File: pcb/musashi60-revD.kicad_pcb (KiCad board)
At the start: 2 copper layers, 160 x 135 mm, 68 parts, among them J1 MJ-4PP-9, U1 ProMicro_r

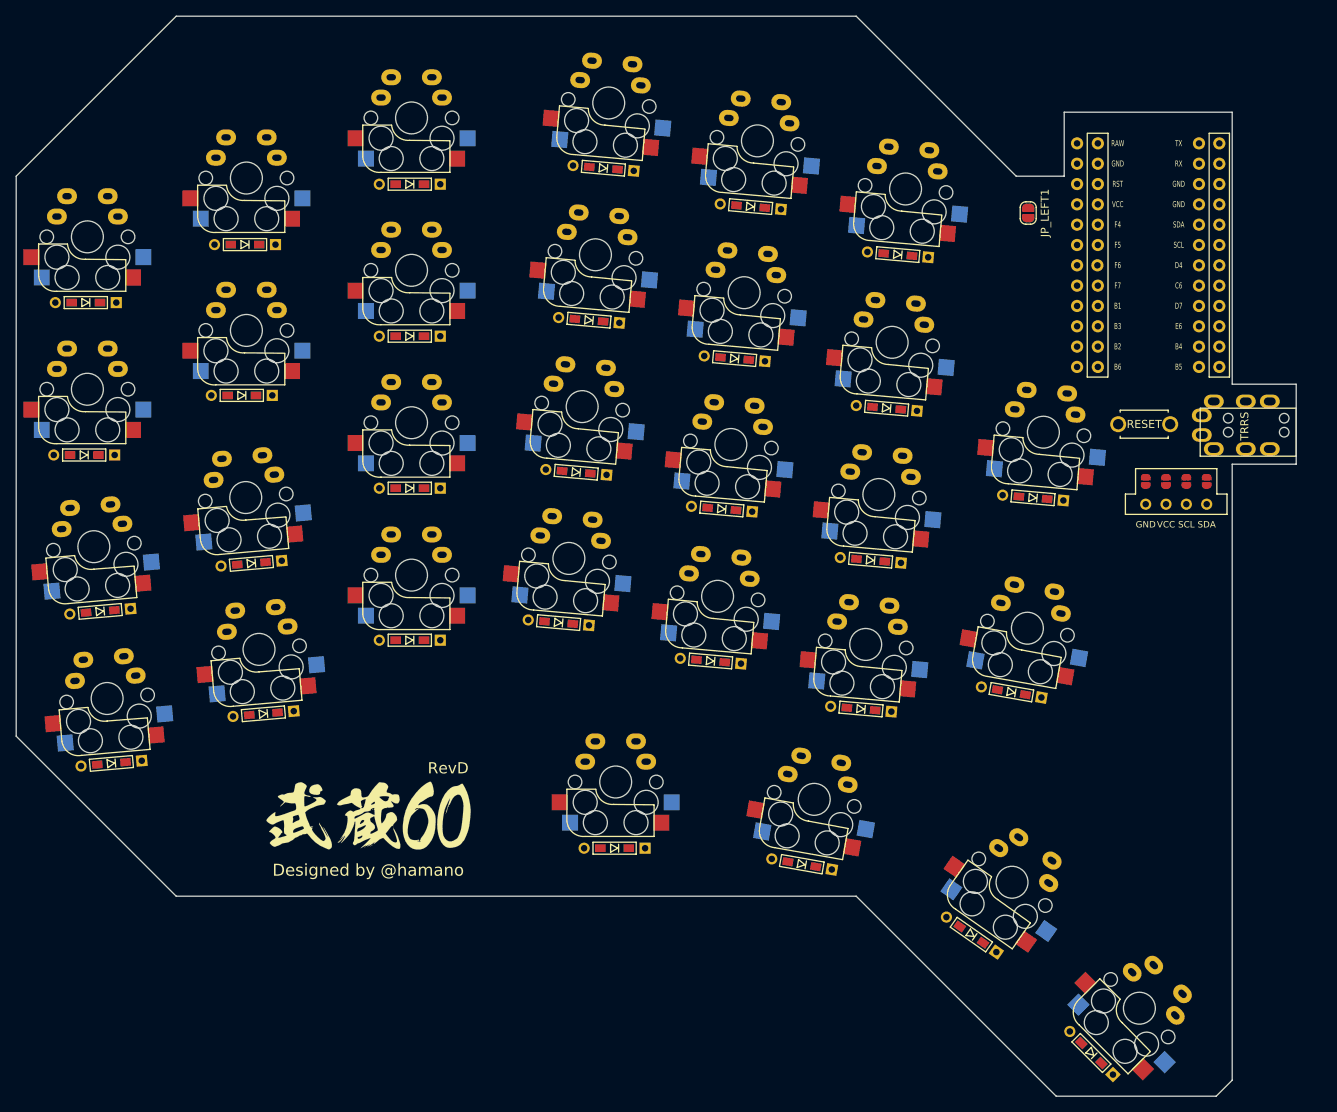
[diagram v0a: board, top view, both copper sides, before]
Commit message: update revD pcb
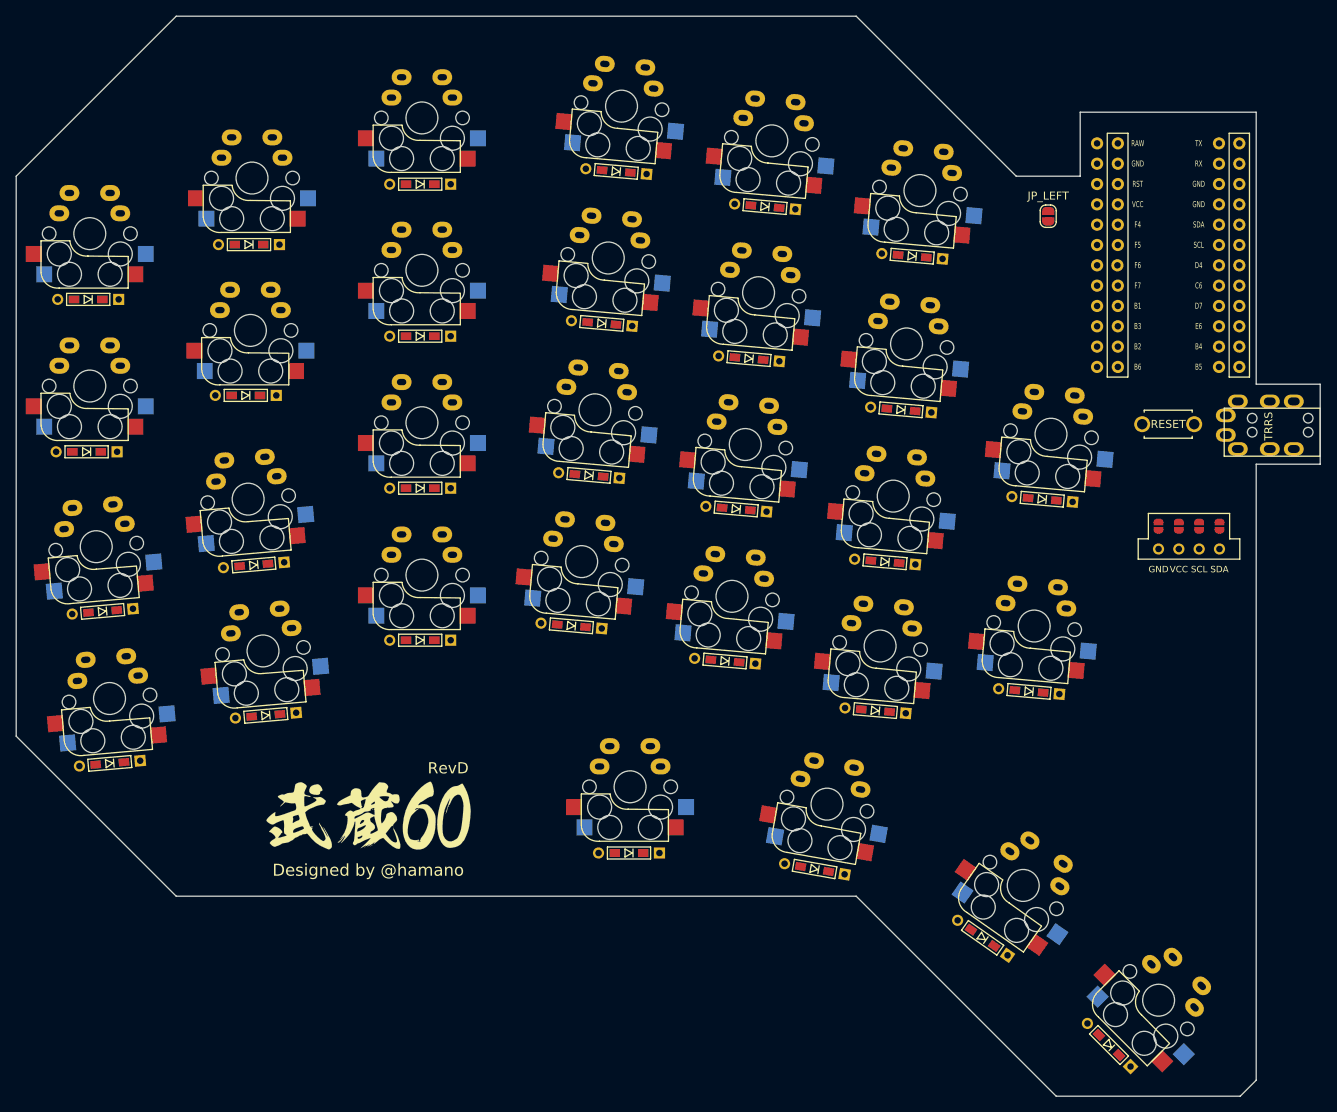
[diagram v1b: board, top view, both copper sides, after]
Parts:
- JP_LEFT1, JP_RIGHT1: footprint Jumper:SolderJumper-2_P1.3mm_Open_RoundedPad1.0x1.5mm -> local:SolderJumper
- OL1: value OLED_Reversible -> OLED
- SW_RST1: footprint foostan:ResetSW -> local:ResetSW
- moved OL1 5.82 mm to (171.6, 89.6)
- moved J1 3.00 mm to (188.0, 75.0)
- moved SW_RST1 3.00 mm to (169.0, 74.0), turned to 180 degrees
- moved SW_A5 2.60 mm to (167.8, 146.0)
- moved JP_LEFT1 2.53 mm to (154.0, 48.0), turned to 0 degrees
- moved JP_RIGHT1 2.53 mm to (154.0, 48.0), turned to 180 degrees
- moved U1 2.50 mm to (169.0, 51.6)
- moved D_A5 2.42 mm to (161.6, 151.6)
- moved D_A3 2.20 mm to (151.6, 107.4), turned to 175 degrees
- moved SW_D5 1.90 mm to (101.7, 119.3)
- moved D_D5 1.90 mm to (101.6, 127.6)
- moved D_B1 1.81 mm to (137.0, 53.0)
- moved D_B4 1.81 mm to (132.4, 109.8)
- moved SW_B3 1.81 mm to (134.6, 83.0)
- moved SW_B4 1.81 mm to (133.0, 101.7)
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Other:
- board size 160 x 135 mm -> 163 x 135 mm
